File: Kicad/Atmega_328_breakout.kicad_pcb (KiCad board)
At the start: 2 copper layers, 73.8 x 62 mm, 71 parts, among them J1 Jack-DC, J10 Conn_01x06, J11 01x03, J12 01x03, J13 01x03, J14 01x03, J15 01x03, J16 01x03, J17 01x03, J18 01x03, J19 Power_connector, J2 01x03, J20 ADC_Connector, J21 PORB++_connector, J22 PORD_connector, J23 Conn_01x01, J24 Device_Connector, J25 Pin out, J26 Com_header, J27 Power terminal, J28 USB, J3 01x03, J4 01x03, J5 01x03, J6 01x03, J7 01x03, J8 01x03, J9 01x03, Q1 PMOS, SW1 SW_Push, SW2 SW_Push, U1 NCP1117-5, U2 L7805, U3 LM358, U4 ATMEGA328P-AU, U5 MCP1700-33, U6 MCP2221, Y1 Crystal_GND24

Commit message: Release-2.0
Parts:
- D3: value LED -> LED on
- D4: value LED -> LED user

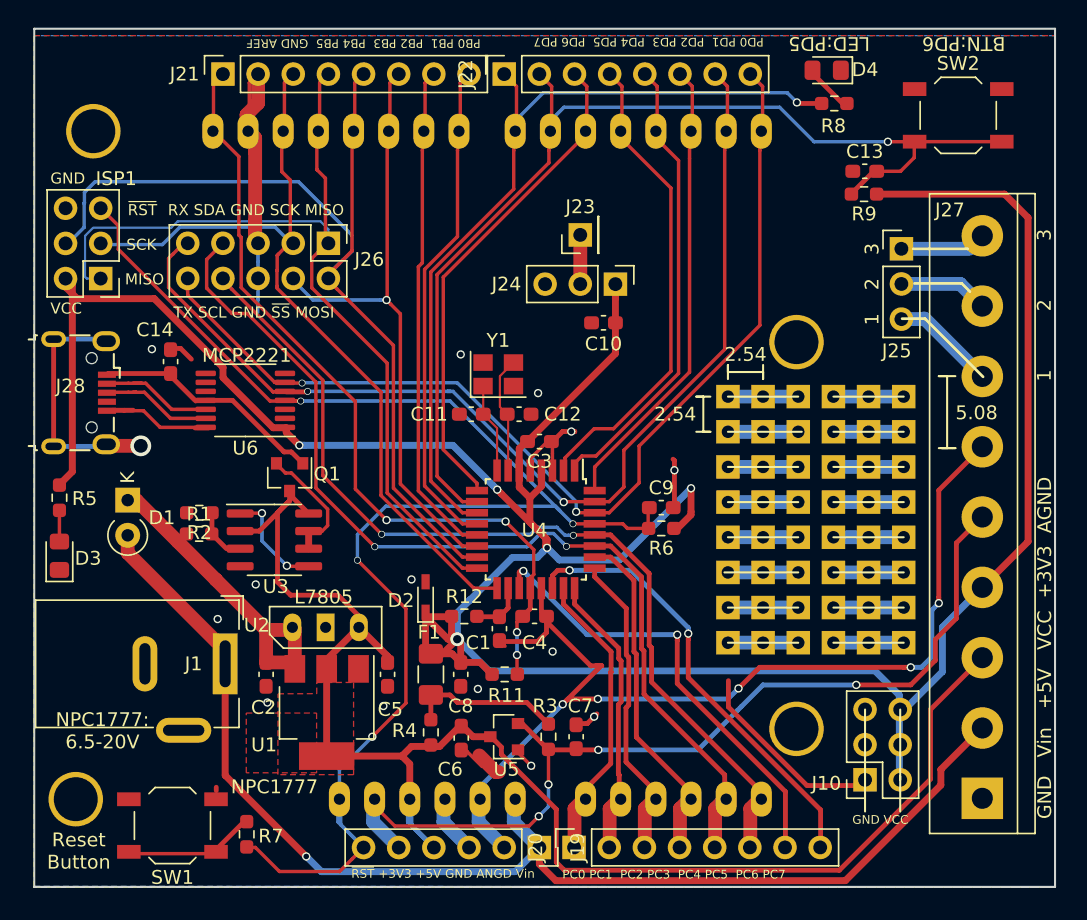
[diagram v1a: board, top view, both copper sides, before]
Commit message: started adding new parts
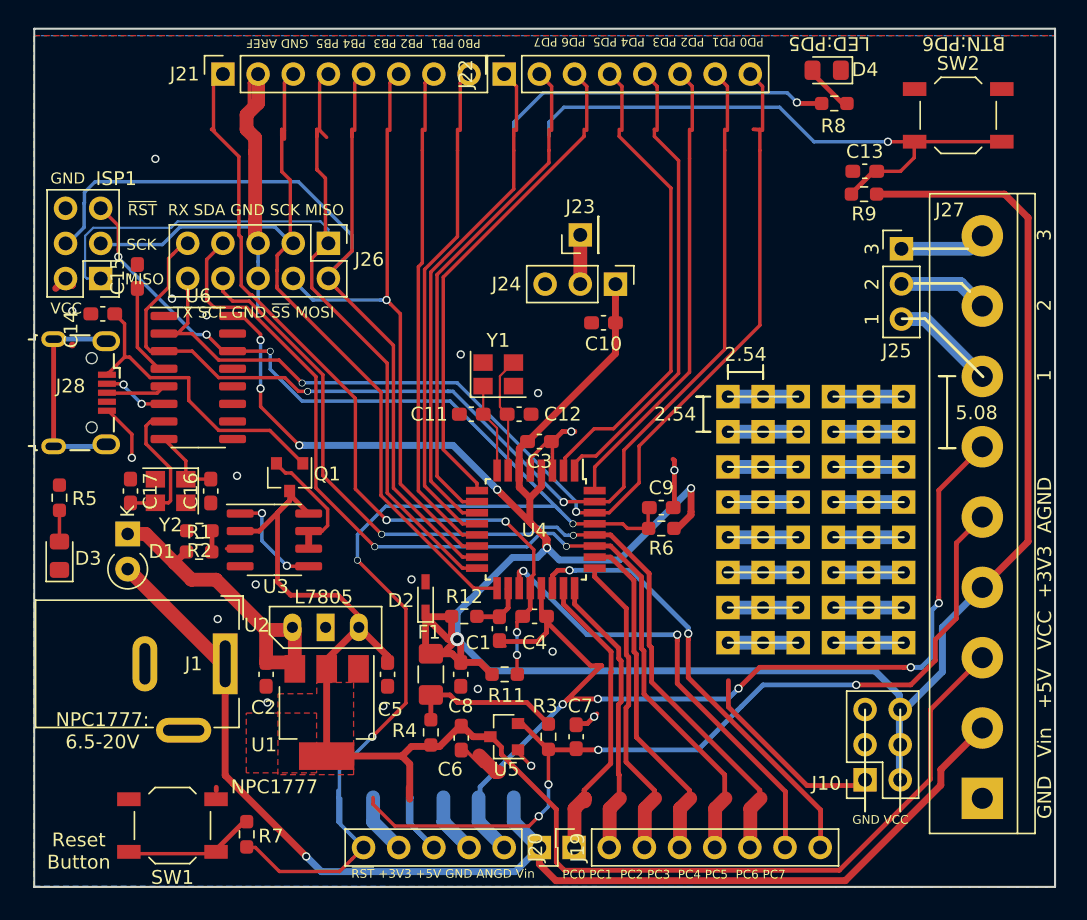
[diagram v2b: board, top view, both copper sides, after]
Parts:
- removed SHIELD1: ATMEL_SHIELD, jorgen:AtmelSHIELD
- added C15: 100n, Capacitor_SMD:C_0603_1608Metric_Pad1.08x0.95mm_HandSolder, F.Cu at (57.7, 71.9)
- added C16: 33p, Capacitor_SMD:C_0603_1608Metric_Pad1.08x0.95mm_HandSolder, F.Cu at (63.0, 87.4)
- added C17: 33p, Capacitor_SMD:C_0603_1608Metric_Pad1.08x0.95mm_HandSolder, F.Cu at (57.2, 87.4)
- added Y2: Crystal_GND24_12MHz, Crystal:Crystal_SMD_3225-4Pin_3.2x2.5mm, F.Cu at (60.1, 87.4)
- U6: value MCP2221 -> CH340G; footprint Package_SO:TSSOP-14_4.4x5mm_P0.65mm -> Package_SO:SOIC-16_3.9x9.9mm_P1.27mm
- Y1: value Crystal_GND24 -> Crystal_GND24_16MHz
- moved C14 5.99 mm to (55.2, 74.6), turned to 0 degrees
- moved U6 3.78 mm to (62.1, 79.2), turned to 0 degrees
- moved D1 2.44 mm to (57.0, 90.5)
- moved R1 1.30 mm to (62.2, 91.8)
- moved R2 1.30 mm to (62.2, 90.3)
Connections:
- U6 pad 1: VCC -> GND
- U6 pad 11: VUSB -> Net-(U6-Pad11)
- U6 pad 12: Net-(J28-Pad2) -> Net-(U6-Pad12)
- U6 pad 13: Net-(J28-Pad3) -> Net-(U6-Pad13)
- U6 pad 14: GND -> ~RESET
- U6 pad 2: Net-(U6-Pad2) -> PD0(RX)
- U6 pad 3: Net-(U6-Pad3) -> PD1(TX)
- U6 pad 4: ~RESET -> Net-(C15-Pad1)
- U6 pad 5: PD1(TX) -> Net-(J28-Pad3)
- U6 pad 6: PD0(RX) -> Net-(J28-Pad2)
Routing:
- net VCC: track 224.9 -> 200.6 mm, vias 5 -> 7
- net Net-(C17-Pad2): track 0.00 -> 10.5 mm
- net GND: track 77.6 -> 69.8 mm, vias 14 -> 19
- net Net-(C15-Pad1): track 0.00 -> 6.82 mm
- net VUSB: track 16.2 -> 22.4 mm
- net Net-(C16-Pad2): track 0.00 -> 5.36 mm
- net PD0(RX): track 78.0 -> 83.3 mm
- net PD1(TX): track 77.1 -> 81.9 mm
- net Net-(J28-Pad3): track 7.47 -> 4.34 mm
- net Net-(J28-Pad2): track 7.87 -> 4.79 mm, vias 0 -> 2
- net Net-(J28-Pad6): track 18.2 -> 15.6 mm, vias 1 -> 0
- net Net-(R1-Pad2): track 4.03 -> 2.52 mm
- net V_supply: track 89.9 -> 88.5 mm
- net ~RESET: track 108.9 -> 110.1 mm, vias 4 -> 6
- net Net-(C2-Pad2): track 25.6 -> 24.6 mm
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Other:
- board text removed: "MCP2221"
